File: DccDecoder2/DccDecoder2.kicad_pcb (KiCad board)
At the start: 2 copper layers, 94 x 35.6 mm, 33 parts, among them IC1 AP64060QWU-7, J1 DCC, J2 0, J3 1, J4 2, J5 3, J6 +V, J7 M_OUT_B, J8 M_OUT_A, J9 GND, Q1 T2N7002BK, Q2 T2N7002BK, Q3 T2N7002BK, Q4 T2N7002BK, Q5 T2N7002BK, SW1 SW_Push, U1 Pico, U2 BDR6133

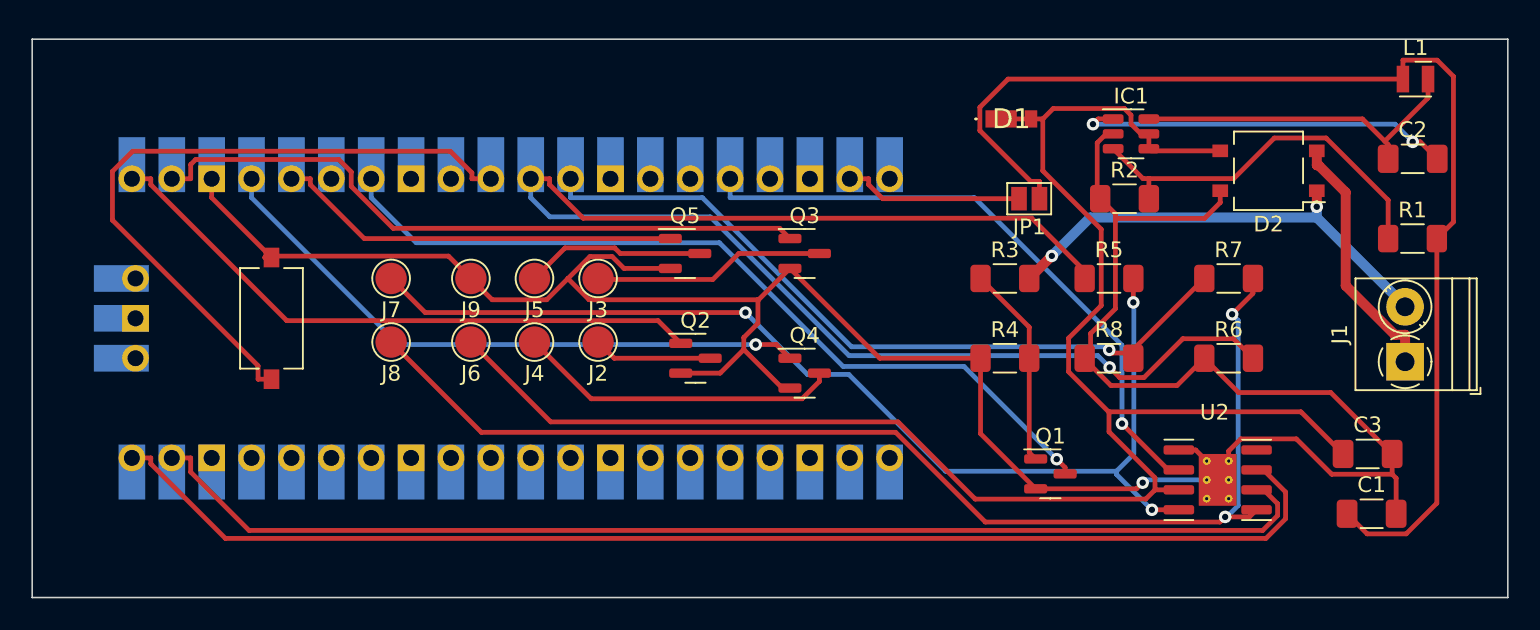
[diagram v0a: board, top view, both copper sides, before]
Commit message: 04/12/24 22:17 Titan.local
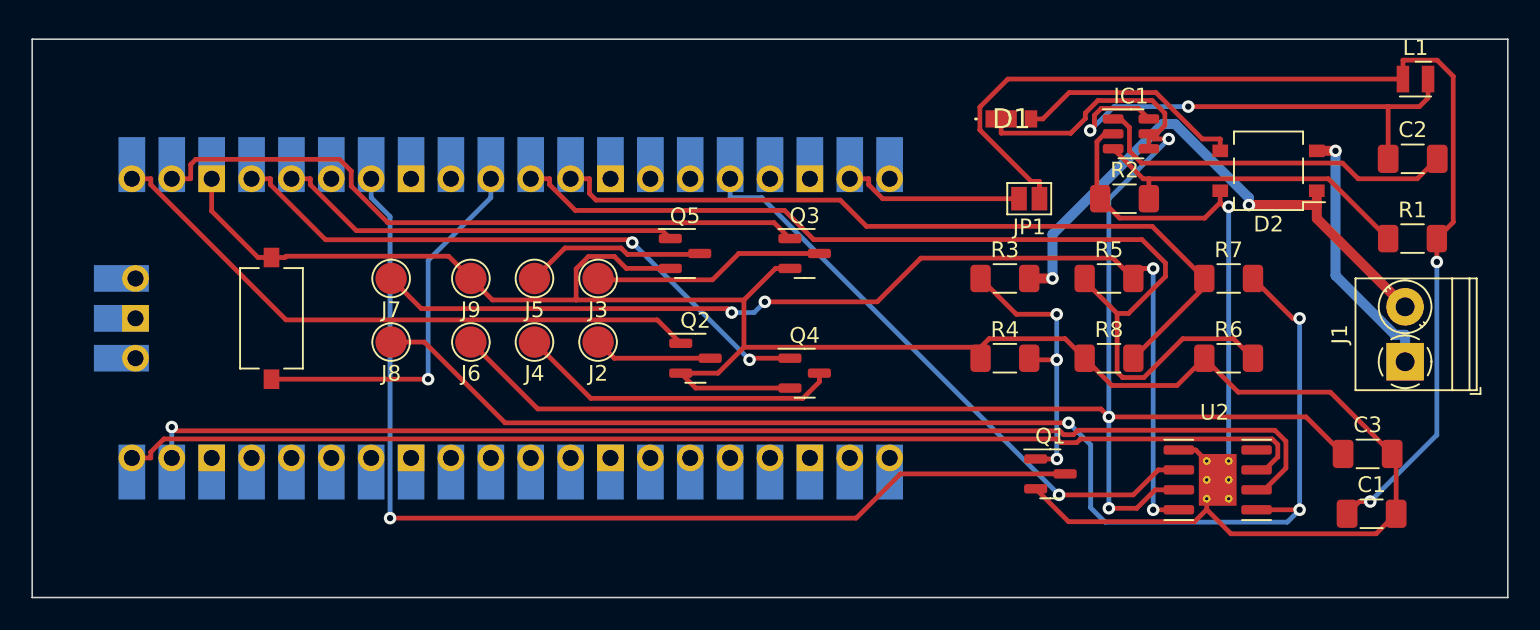
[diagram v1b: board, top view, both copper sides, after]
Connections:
- D1 pad 2: +V -> Net-(D1-A)
- D2 pad 3: +V -> Net-(D1-A)
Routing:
- net /ADC_EMF_A: track 91.9 -> 64.9 mm, vias 1 -> 0
- net Net-(U1-RUN): track 43.5 -> 24.4 mm, vias 0 -> 1
- net Net-(D1-A): track 0.00 -> 14.7 mm
- net /GPIO21: track 52.9 -> 66.3 mm
- net GND: track 171.3 -> 182.5 mm
- net Net-(IC1-SW): track 21.9 -> 31.9 mm, vias 0 -> 2
- net /MOTOR_OUT_B: track 76.5 -> 84.2 mm, vias 2 -> 3
- net Net-(J1-Pin_2): track 29.6 -> 36.2 mm
- net Net-(Q1-G): track 13.0 -> 18.2 mm, vias 0 -> 3
- net +V: track 110.0 -> 105.7 mm, vias 0 -> 3
- net /GPIO15: track 80.5 -> 76.5 mm
- net /5V: track 74.9 -> 71.3 mm, vias 0 -> 2
- net Net-(IC1-FB): track 24.7 -> 21.2 mm
- net /ADC_EMF_B: track 48.1 -> 50.5 mm, vias 1 -> 0
- net /GPIO14: track 75.7 -> 77.7 mm, vias 0 -> 1
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
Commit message: 09/12/24 17:09 Arrakis.local
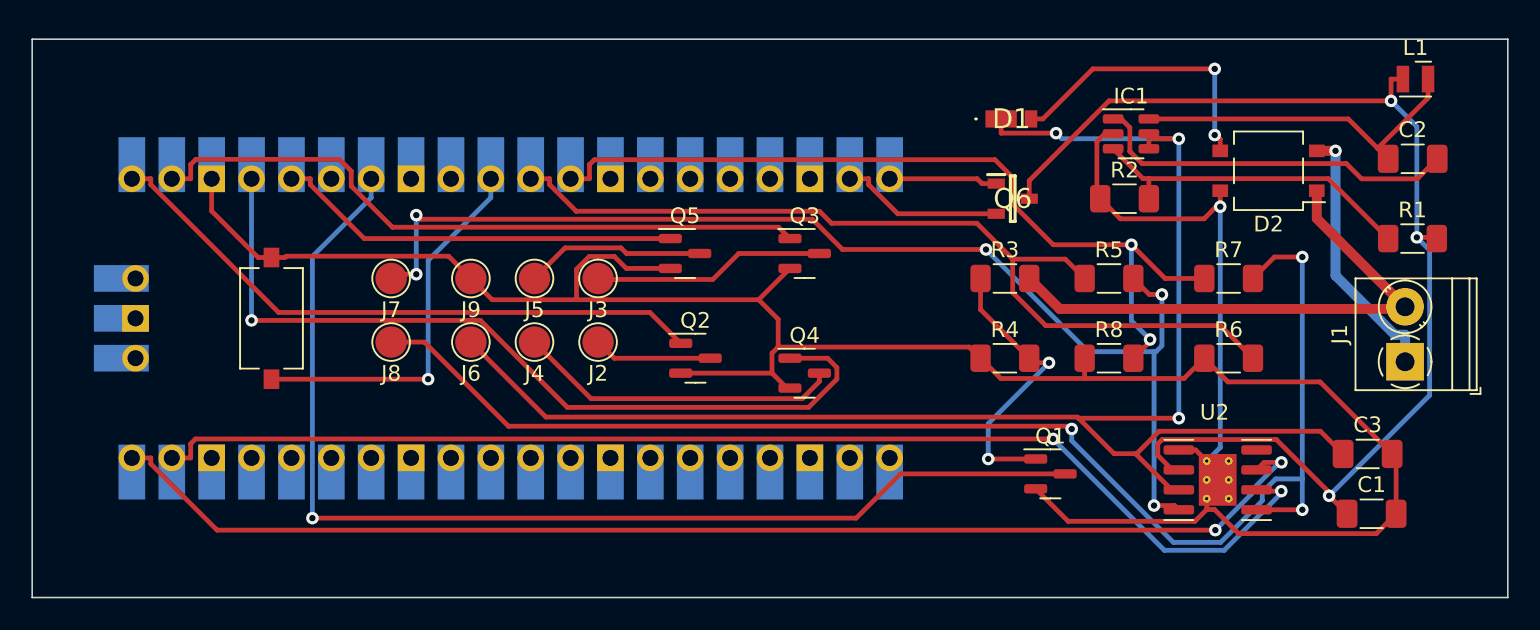
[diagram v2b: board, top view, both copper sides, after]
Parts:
- removed JP1: Jumper_2_Open, Jumper:SolderJumper-2_P1.3mm_Open_Pad1.0x1.5mm
- added Q6: DMG2305UX-7, DMG2305UX-7:SOT96P240X110-3N, F.Cu at (161.5, 58.4)
- R1: value 115k -> 69k8
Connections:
- C1 pad 1: /5V -> +3V3
- L1 pad 1: /5V -> +3V3
- R1 pad 2: /5V -> +3V3
- U1 pad 36: +3V3 -> unconnected-(U1-3V3-Pad36)
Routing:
- net /5V: track 71.3 -> 0.00 mm, vias 2 -> 0
- net +3V3: track 38.3 -> 75.3 mm, vias 1 -> 3
- net /GPIO18: track 39.3 -> 53.3 mm, vias 2 -> 1
- net Net-(IC1-SW): track 31.9 -> 22.0 mm, vias 2 -> 0
- net /ADC_EMF_A: track 64.9 -> 57.3 mm
- net unconnected-(Q6-Pad1): track 0.00 -> 6.92 mm
- net /GPIO21: track 66.3 -> 72.3 mm
- net /MOTOR_OUT_A: track 68.7 -> 73.7 mm, vias 4 -> 5
- net GND: track 182.5 -> 177.6 mm
- net /MOTOR_OUT_B: track 84.2 -> 88.5 mm
- net Net-(D1-A): track 14.7 -> 18.4 mm, vias 0 -> 2
- net /ADC_EMF_B: track 50.5 -> 53.7 mm, vias 0 -> 2
- net +V: track 105.7 -> 102.9 mm
- net /GPIO15: track 76.5 -> 79.0 mm, vias 0 -> 2
- net Net-(J1-Pin_2): track 36.2 -> 34.5 mm, vias 2 -> 0
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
